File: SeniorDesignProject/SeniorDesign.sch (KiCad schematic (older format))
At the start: 27 parts, among them J1 RJ45(LoadCells), J2 RJ45(Accelerometer), J3 PICkit3, J4 RJ11(ICD3), J5 ID-12LA Header, J6 XBEE Header, J7 7-Segment Display, P7 Power 1, P9 Power 2, U1 INA827, U10 7905, U9 7805

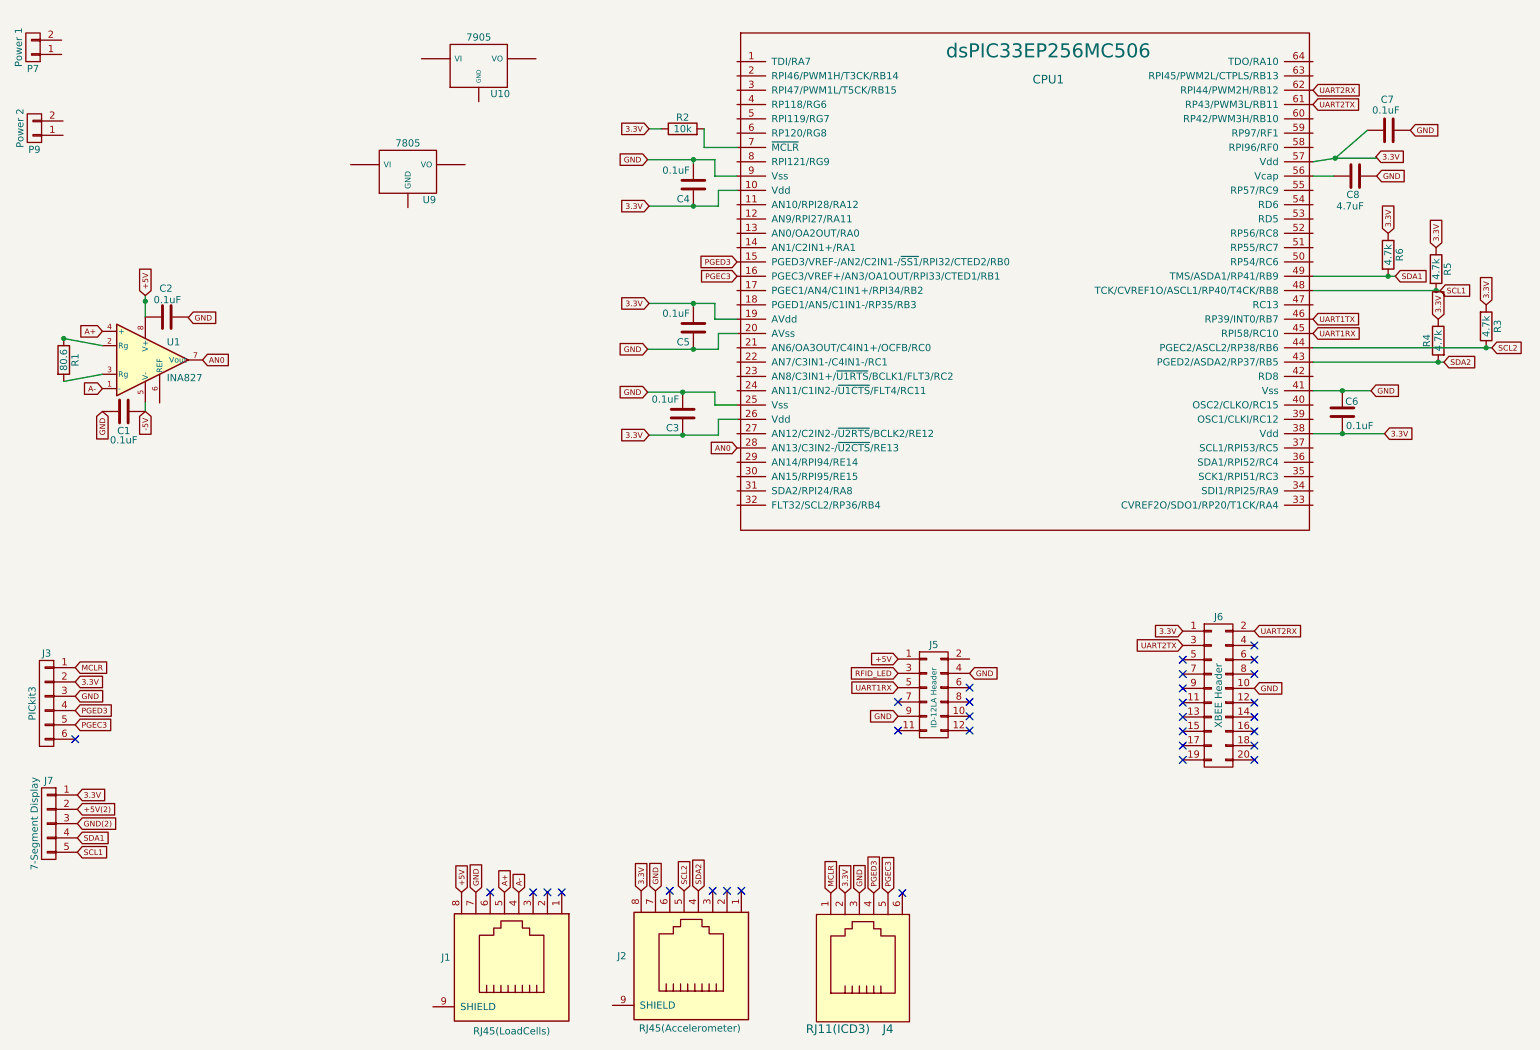
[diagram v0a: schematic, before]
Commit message: Updates to board
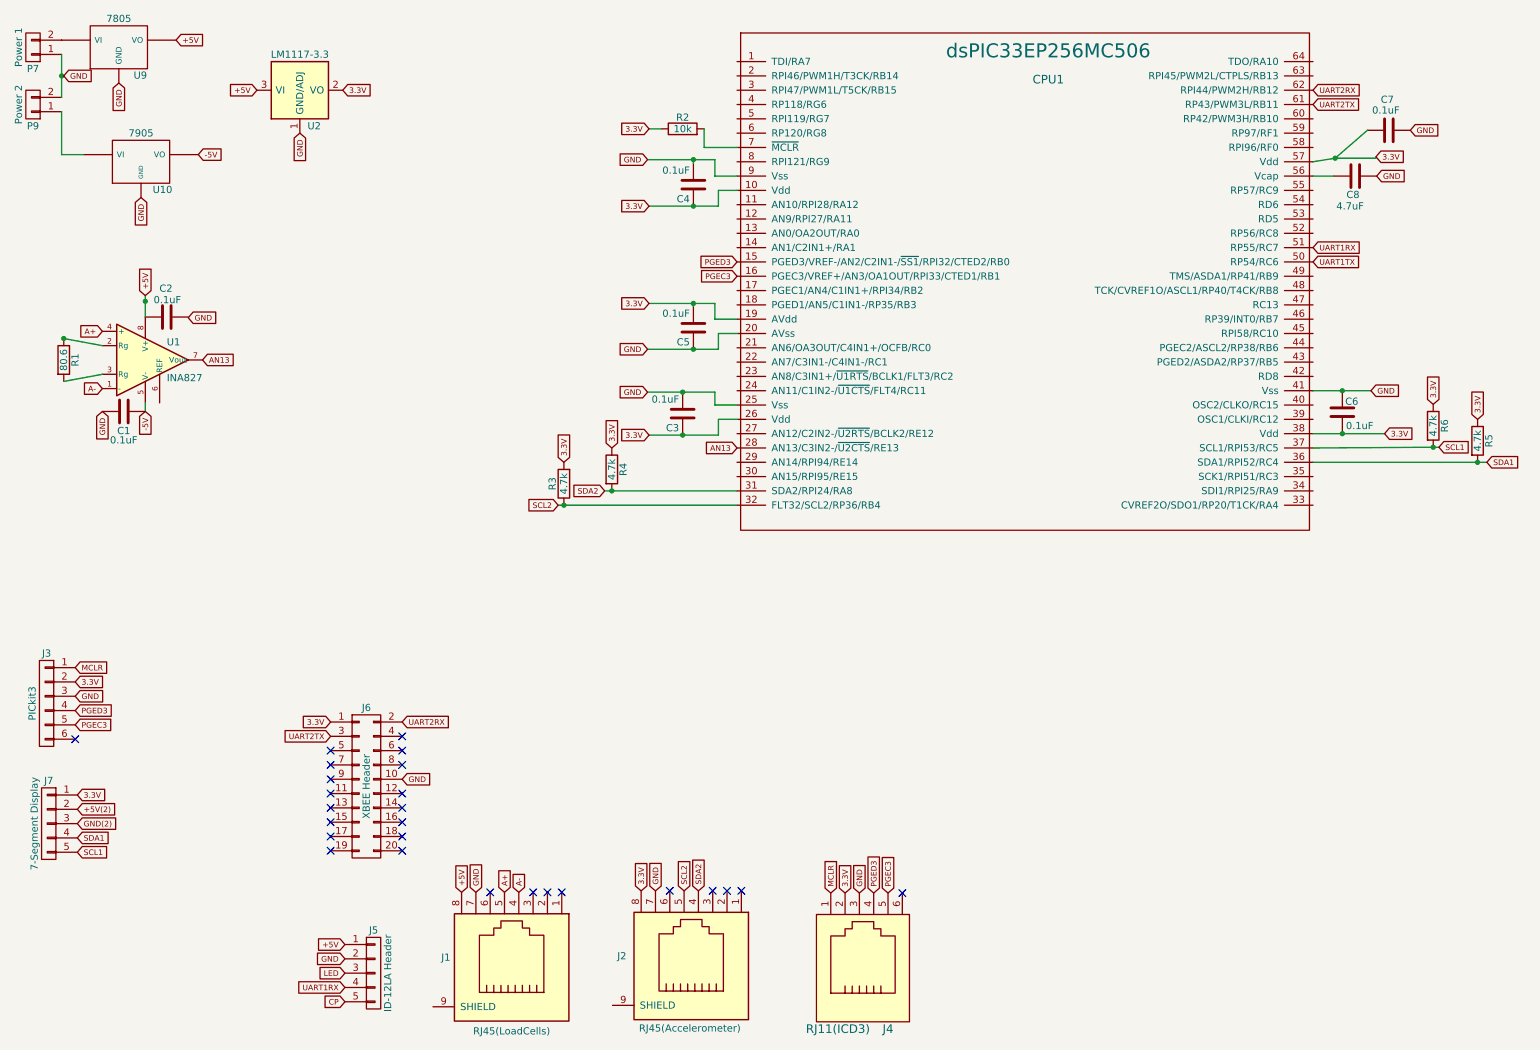
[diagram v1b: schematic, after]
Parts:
- removed J5: ID-12LA Header, Pin_Headers:Pin_Header_Straight_2x06_Pitch2.54mm, symbol CONN_02X06
- added J5: ID-12LA Header, Socket_Strips:Socket_Strip_Straight_1x05_Pitch2.54mm, symbol CONN_01X05
- added U2: LM1117-3.3, TO_SOT_Packages_SMD:SOT-223, symbol LM1117-3.3
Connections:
- net +5V: now also U9.VO, J5.1 (P1), U2.3 (VI)
- net -5V: now also U10.VO
- net 3.3V: now also U2.2 (VO), U2.4 (VO)
- net GND: now also P7.1 (P1), P9.2 (P2), U10.GND, U9.GND, J5.2 (P2), U2.1 (GND/ADJ)
- net SCL1: now also CPU1.37 (SCL1/RPI53/RC5), R6.2; no longer CPU1.48 (TCK/CVREF1O/ASCL1/RP40/T4CK/RB8), R5.2
- net SCL2: now also CPU1.32 (FLT32/SCL2/RP36/RB4); no longer CPU1.44 (PGEC2/ASCL2/RP38/RB6)
- net SDA1: now also CPU1.36 (SDA1/RPI52/RC4), R5.2; no longer CPU1.49 (TMS/ASDA1/RP41/RB9), R6.2
- net SDA2: now also CPU1.31 (SDA2/RPI24/RA8); no longer CPU1.43 (PGED2/ASDA2/RP37/RB5)
- net UART1RX: now also CPU1.51 (RP55/RC7), J5.4 (P4); no longer CPU1.45 (RPI58/RC10)
- net UART1TX: now also CPU1.50 (RP54/RC6); no longer CPU1.46 (RP39/INT0/RB7)
- net at P7.2 (P2): now also U9.VI
- net at U10.VI: now also P9.1 (P1)
- net AN0 renamed AN13
- new net CP: J5.5 (P5)
- new net LED: J5.3 (P3)
- no-connect marks 32 -> 26
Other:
- moved on the sheet: J6, P9, R3, R4, R5, R6, U10, U9
